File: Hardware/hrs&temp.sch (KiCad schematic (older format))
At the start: 26 parts, among them IC1 AP7366-33SN-7, J3 Conn_01x02, U2 PAH8011-ETLGA, U3 TP4057X, U5 SGM2031-1.8YUDH4G/TR

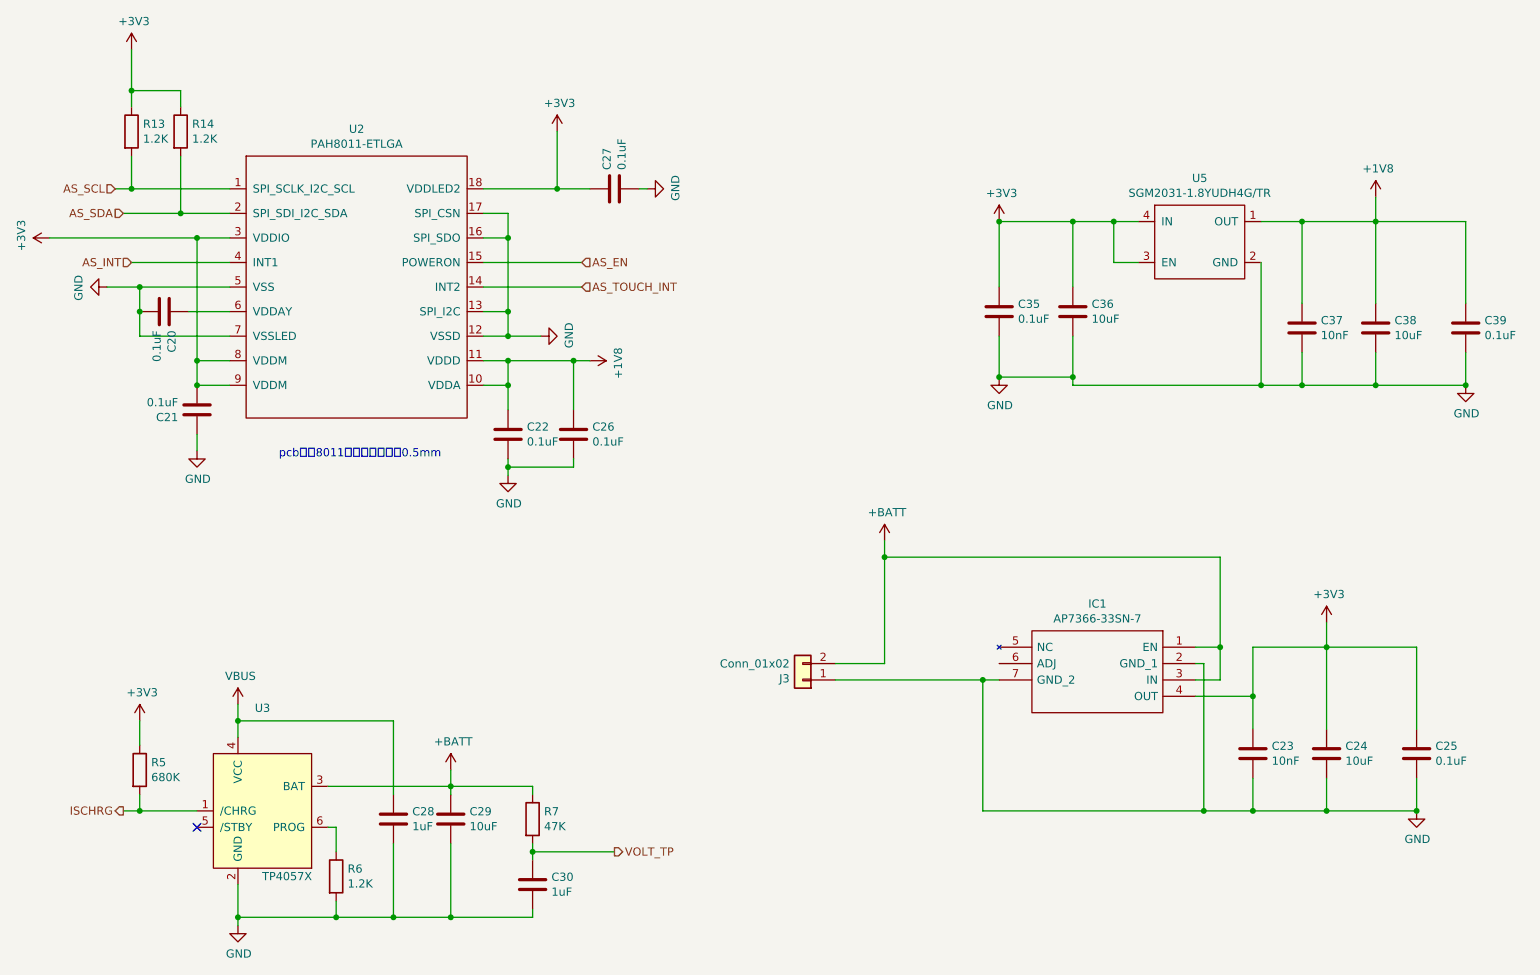
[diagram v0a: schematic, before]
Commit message: xiaoming-opensource
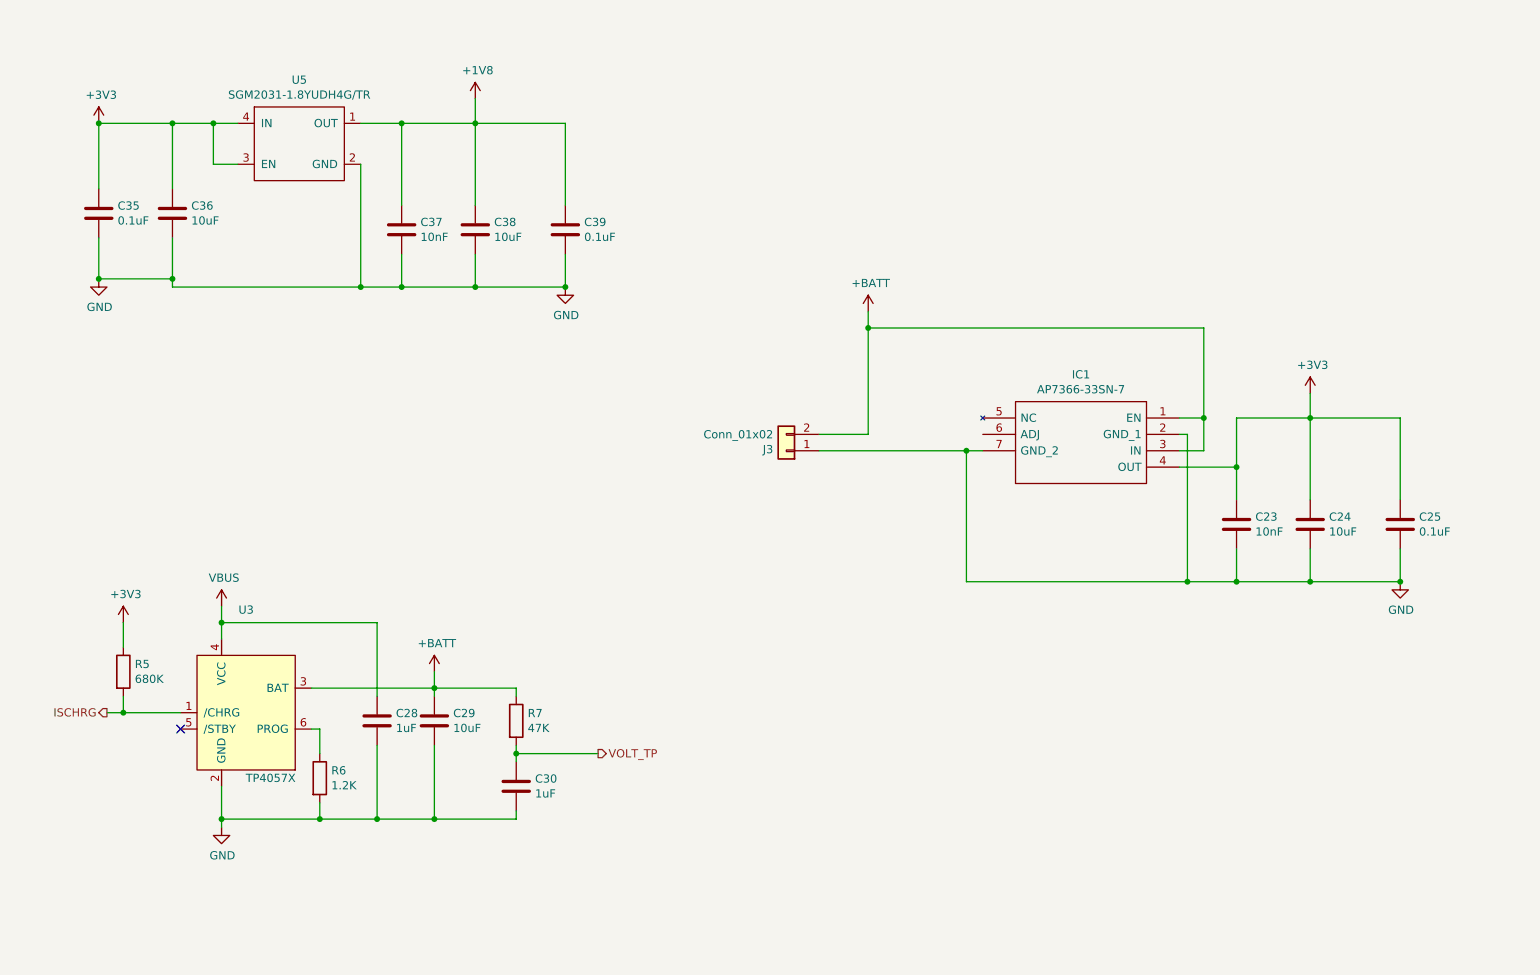
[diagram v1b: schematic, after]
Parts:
- removed C20, C21, C22, C26, C27: 0.1uF, Capacitor_SMD:C_0402_1005Metric, symbol Medical_Ring-v5.2-rescue:C-Device
- removed R13, R14: 1.2K, Resistor_SMD:R_0402_1005Metric, symbol Medical_Ring-v5.2-rescue:R-Device
- removed U2: PAH8011-ETLGA, Package_DFN_QFN:PAH8011ET, symbol Medical_Ring-v5.2-rescue:PAH8011-ETLGA-Sensor_Optical
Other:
- note removed: "pcb中，8011位置有意左偏移0.5mm"
- moved on the sheet: C23, C24, C25, C28, C29, C30, C35, C36, C37, C38, C39, IC1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
